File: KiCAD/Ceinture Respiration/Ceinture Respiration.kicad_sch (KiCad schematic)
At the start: 2 parts, among them J1 Conn_01x10_Pin, J2 Conn_01x10_Socket

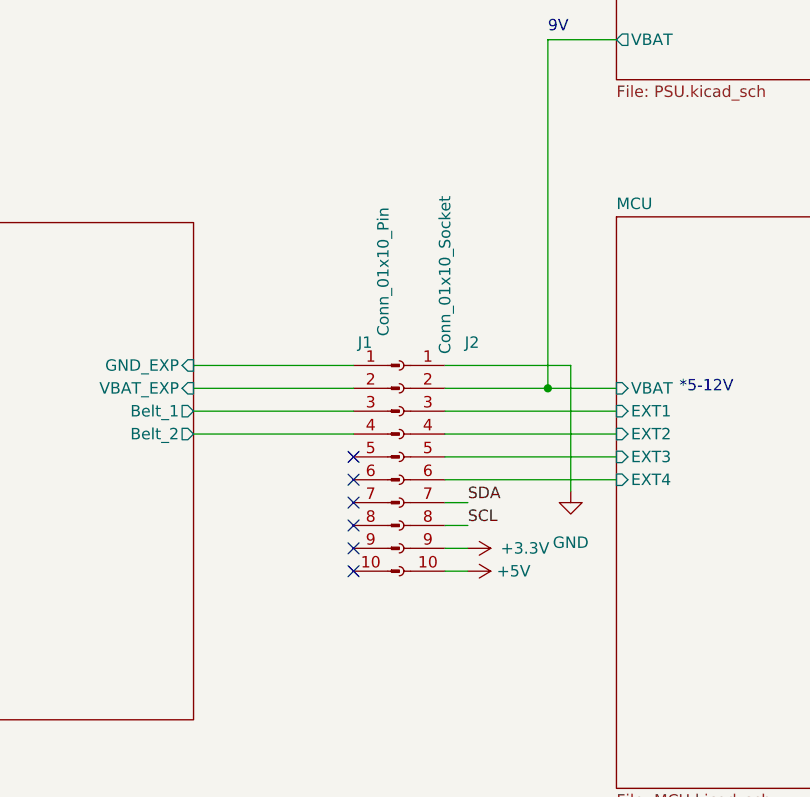
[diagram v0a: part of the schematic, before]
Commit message: sch 99% pcb 99%
Reste à préparer les commandes
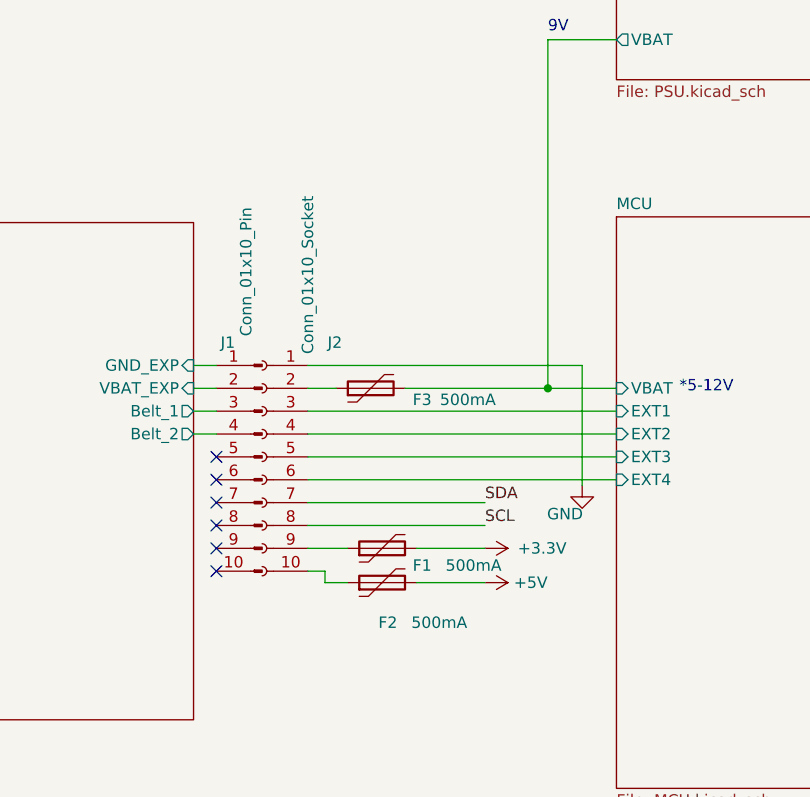
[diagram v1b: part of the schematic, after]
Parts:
- added F1, F2, F3: 500mA, Fuse:Fuse_0603_1608Metric, symbol Device:Polyfuse
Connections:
- net +3.3V: now also F1.2; no longer J2.9 (Pin_9)
- net +5V: now also F2.2; no longer J2.10 (Pin_10)
- net BATTERIE 9V/VBAT: now also F3.2; no longer J2.2 (Pin_2)
- new net: F2.1, J2.10 (Pin_10)
- new net: F3.1, J2.2 (Pin_2)
- new net: F1.1, J2.9 (Pin_9)
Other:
- moved on the sheet: J1, J2

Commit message: PCB sent for production
See latest production files.
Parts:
- F1, F2, F3: LCSC (none) -> C2844464
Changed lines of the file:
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@@
+      (effects (font (size 1.27 1.27)) hide)
+    )
+    (property "LCSC" "C2844464" (at 137.16 118.745 0)
       (effects (font (size 1.27 1.27)) hide)
     )
@@
     )
     (property "Datasheet" "~" (at 135.89 97.155 0)
+      (effects (font (size 1.27 1.27)) hide)
+    )
+    (property "LCSC" "C2844464" (at 135.89 97.155 90)
       (effects (font (size 1.27 1.27)) hide)
     )
@@
       (effects (font (size 1.27 1.27)) hide)
     )
+    (property "LCSC" "C2844464" (at 137.16 114.935 0)
+      (effects (font (size 1.27 1.27)) hide)
+    )
